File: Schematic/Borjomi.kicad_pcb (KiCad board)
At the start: 2 copper layers, 10 parts, among them J1 Vin 12V, J2 Vout 12V, J3 Water Switch 12V, J4 Data in, J5 Data out, J6 Conn_01x02, U1 MCP2515-TJA1050, U2 MH-Series, U3 5V_Relay_Module

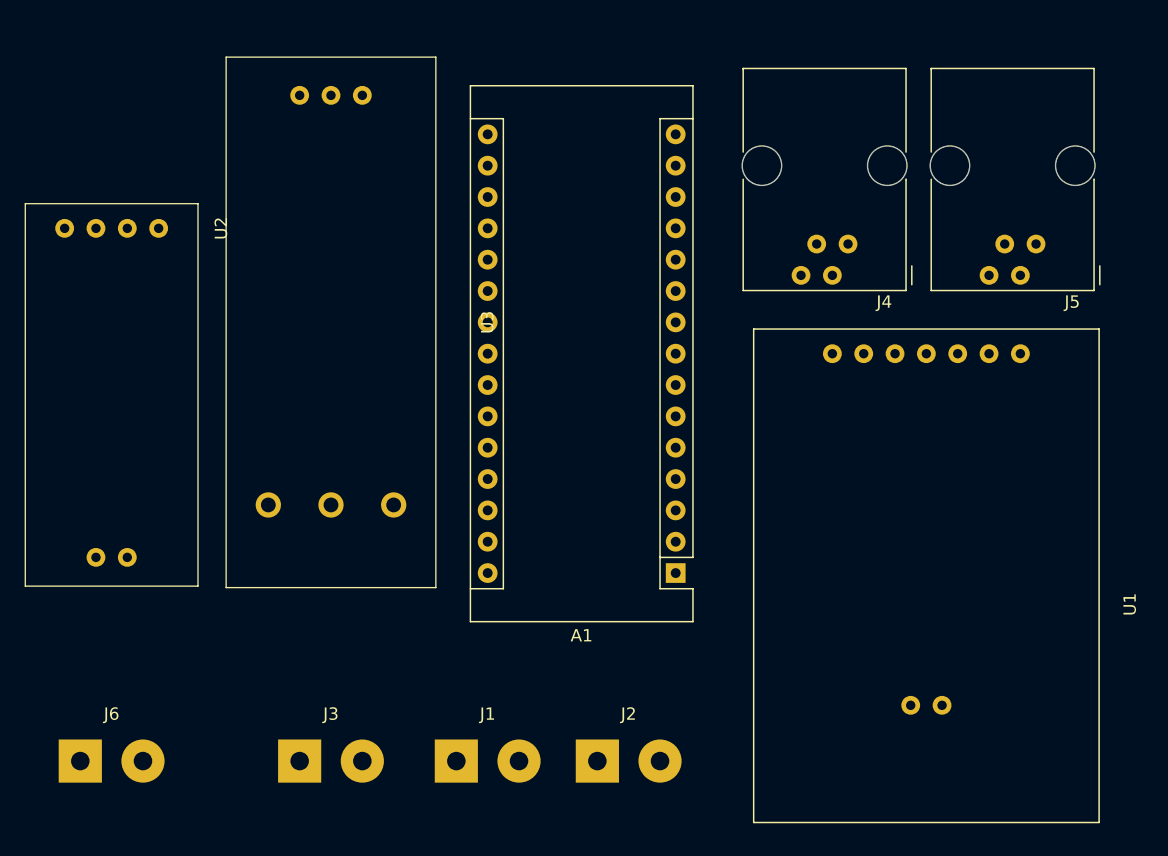
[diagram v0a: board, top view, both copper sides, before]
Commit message: Pcb v1.0 + gerber files
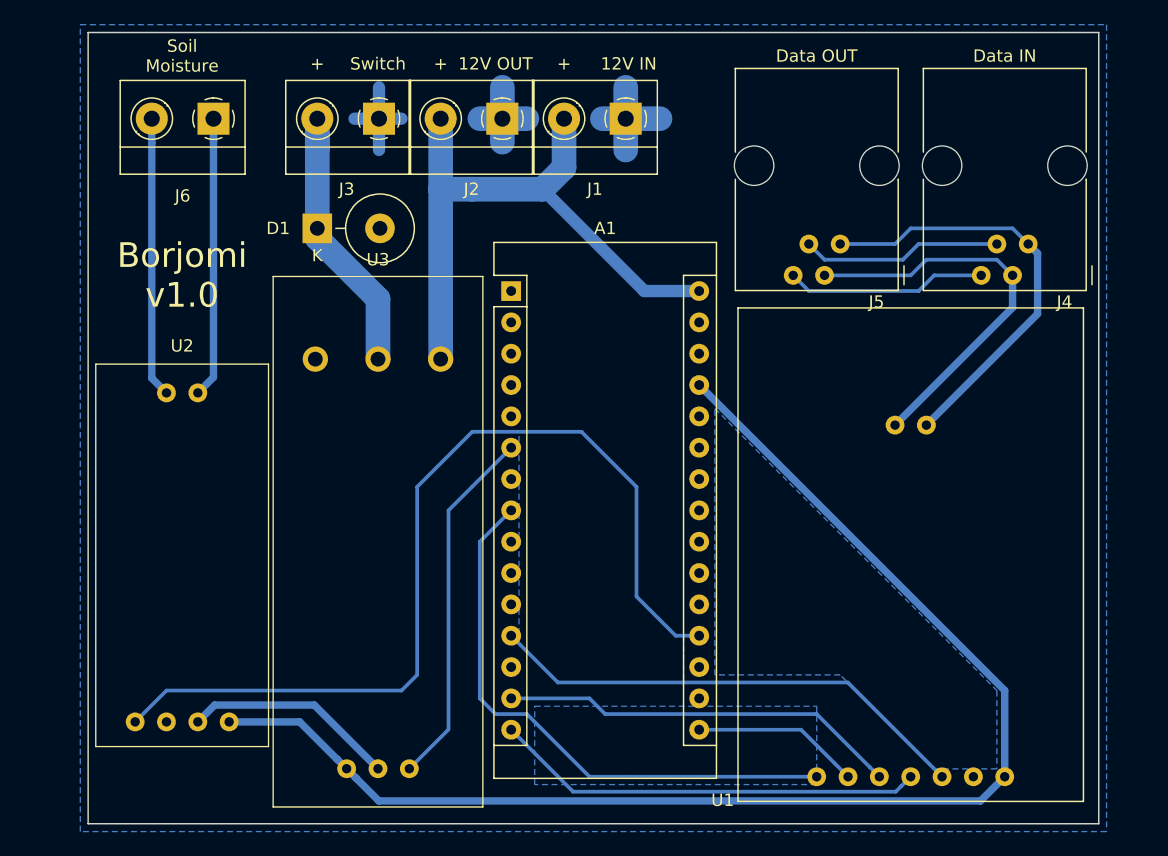
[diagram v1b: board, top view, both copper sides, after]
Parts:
- added D1: 1N5408, Diode_THT:D_DO-27_P5.08mm_Vertical_KathodeUp, F.Cu at (67.5, 50.8)
- J1, J2, J3, J6: footprint Connector_Wire:SolderWirePad_1x02_P5.08mm_Drill1.5mm -> Connector:Degson_DG301_1x02_P5.00mm_Horizontal
- moved J1 53.8 mm to (92.5, 41.9), turned to 180 degrees
- moved J6 53.2 mm to (59.1, 41.9), turned to 180 degrees
- moved J2 52.6 mm to (82.5, 41.9), turned to 180 degrees
- moved J3 52.5 mm to (72.5, 41.9), turned to 180 degrees
- moved U2 40.4 mm to (56.5, 90.8), turned to 90 degrees
- moved U1 34.3 mm to (115.6, 95.2), turned to 90 degrees
- moved A1 26.5 mm to (83.2, 55.9), turned to 0 degrees
- moved U3 18.2 mm to (72.4, 76.2), turned to 90 degrees
- moved J5 15.9 mm to (111.1, 54.6)
- moved J4 14.6 mm to (126.4, 54.6)
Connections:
- A1 pad 5: Net-(A1-Pad5) -> (no net)
- A1 pad 8: (no net) -> Net-(A1-Pad8)
- J3 pad 1: Net-(J3-Pad1) -> GND
- J3 pad 2: GND -> Net-(D1-Pad1)
- U1 pad 1: Net-(J4-Pad2) -> Net-(J4-Pad1)
- U1 pad 2: Net-(J4-Pad1) -> Net-(J4-Pad2)
- U1 pad 3: Net-(A1-Pad5) -> Net-(A1-Pad8)
- U2 pad 5: Net-(J6-Pad2) -> Net-(J6-Pad1)
- U2 pad 6: Net-(J6-Pad1) -> Net-(J6-Pad2)
- U3 pad 4: Net-(J3-Pad1) -> +12V
- U3 pad 5: +12V -> Net-(D1-Pad1)
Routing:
- net Net-(A1-Pad27): track 0.00 -> 108.3 mm
- net Net-(A1-Pad19): track 0.00 -> 76.4 mm
- net +12V: track 0.00 -> 50.3 mm
- net Net-(A1-Pad8): track 0.00 -> 46.2 mm
- net GND: track 0.00 -> 44.2 mm
- net Net-(A1-Pad12): track 0.00 -> 39.7 mm
- net Net-(J4-Pad1): track 0.00 -> 35.0 mm
- net Net-(A1-Pad15): track 0.00 -> 35.0 mm
- net Net-(A1-Pad14): track 0.00 -> 32.5 mm
- net Net-(J4-Pad2): track 0.00 -> 32.4 mm
- net Net-(A1-Pad6): track 0.00 -> 29.4 mm
- net Net-(J6-Pad1): track 0.00 -> 23.4 mm
- net Net-(J6-Pad2): track 0.00 -> 22.7 mm
- net Net-(D1-Pad1): track 0.00 -> 22.6 mm
- net Net-(J4-Pad3): track 0.00 -> 16.3 mm
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- added copper zone on B.Cu, net (none)
- added copper zone on B.Cu, net GND
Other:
- board outline added: 81.9 x 64.1 mm
- board text added: "+"
- board text added: "12V IN"
- board text added: "12V OUT"
- board text added: "Borjomi v1.0"
- board text added: "Data IN"
- board text added: "Data OUT"
- board text added: "Soil Moisture"
- board text added: "Switch"
